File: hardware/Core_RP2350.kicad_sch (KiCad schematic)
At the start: 70 parts, among them SW1 SPST-NO, SW2 SPST-NO, SW3 SPST-NO, SW4 SPST-NO, SW5 SPST-NO, U1 RP2350B-QFN80, U2 LM4040A30IDBZR, U3 W25Q128JVS, U4 W25Q128JVS, U5 W25Q128JVS

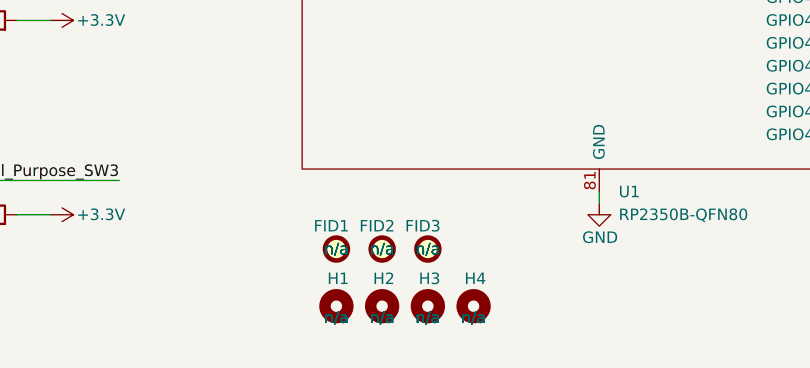
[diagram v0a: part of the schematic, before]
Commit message: The final review has been completed, and the manufacturing files have been generated.
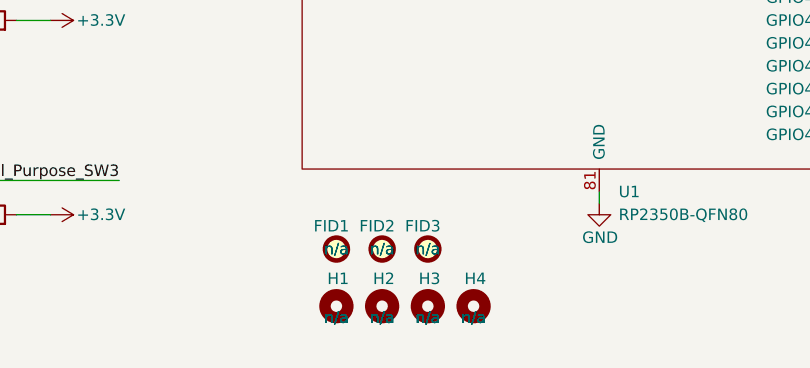
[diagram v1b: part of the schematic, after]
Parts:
- C1, C12, C13, C14, C15, C19, C2, C20, C21, C22, C23, C24, C25, C26, C27, C28, C29, C4, C5, C9: MPN C0603C104K5RACTU -> (none)
- C10, C11, C18: MPN GRM188R61E106KA73D -> (none)
- C16, C17: MPN C1608X5R1V475K080AC -> (none)
- C3: MPN C0603C102K5RACTU -> (none)
- C6: MPN C0603C103K5RACTU -> (none)
- C7, C8: MPN C1608X7R1H105K080AB -> (none)
- FID1, FID2, FID3, H1, H2, H3, H4: MPN n/a -> (none)
- Jump1: MPN M20-9990246 -> (none)
- L1: MPN XGL3530-332MEC -> (none)
- LED1, LED2, LED3: MFN SunLED -> (none); MPN XZCDGK53W-1VF -> (none); Manufacturer_Name SunLED -> Vishay; Manufacturer_Part_Number XZCDGK53W-1VF -> VLMS1300-GS08
- R1: MPN AC0603FR-13100RL -> (none)
- R10, R11: MPN RC0603FR-07220RL -> (none)
- R12: MPN RC0603JR-070RL -> (none)
- R13, R14, R15: MPN RC0603FR-07330RL -> (none)
- R16, R17, R18, R6, R7, R8: MPN RT0603BRD0710KL -> (none)
- R2: MPN RT0603BRD071K1L -> (none)
- R3, R4, R5: MPN AC0603FR-1310RL -> (none)
- R9: MPN AC0603FR-0724RL -> (none)
- SW1, SW2, SW3, SW4, SW5: MFN Würth Elektronik -> (none); MPN 435451019820 -> (none)
- U1: MFN Raspberry Pi -> (none); MPN SC1510-A4 -> (none)
- U2: MPN LM4040A30IDBZR -> (none)
- U3, U4, U5: MPN W25Q128JVSIQ TR -> (none)
- Xtal1: MFN ECS Inc. -> (none); MPN ECS-TXO-2016-33-120-TR -> (none)
